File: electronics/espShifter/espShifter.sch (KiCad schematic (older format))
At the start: 114 parts, among them J1 Power In, J10 12V SENSE, J11 Motor A, J12 Motor E, J13 Motor I, J14 Motor B, J15 Motor F, J16 Motor J, J17 Motor C, J18 Motor G, J19 Motor K, J2 UART, J20 Motor D, J21 Motor H, J22 Motor L, J3 SENSOR, J4 IOVCC, J5 GND, J6 SR CHAIN IN, J7 SR CHAIN OUT, J8 RS485, J9 RS485, Q1 BSS138, Q2 BSS138, U1 Mega2560Shield, U10 ULN2003AModule, U11 INA219 Breakout Wide (blue), U12 ULN2003AModule, U13 ULN2003AModule, U14 ULN2003AModule, U15 ULN2003AModule, U16 LevelShifterModule, U17 RS485Module, U18 TTGO_TDisplay, U19 74HC244, U2 SSD1306_I2C, U20 74HC165, U21 74HC165, U22 ST7789_80x160, U23 D1_32, U24 74HC595, U25 74HC595, U26 74HC595, U27 74HC595, U28 74HC595, U29 74HC595, U3 ULN2003AModule, U30 ST7789_240x240, U31 INA219 Breakout Narrow (purpl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, U32 SP485, U33 INA219BxD, U34 TPL7407LA, U35 TPL7407LA, U36 TPL7407LA, U37 TPL7407LA, U38 TPL7407LA, U39 TPL7407LA, U4 ULN2003AModule, U40 TPL7407LA, U5 ULN2003AModule, U6 ULN2003AModule, U7 ULN2003AModule, U8 ULN2003AModule, U9 ULN2003AModule

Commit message: WIP ESP PCB
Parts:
- removed JP1: 12V_VIN, Connector_PinHeader_2.54mm:PinHeader_1x02_P2.54mm_Vertical, symbol Device:Jumper_NO_Small
- removed R10, R11, R12, R2, R3, R4, R5, R6, R7, R8, R9: 47k, Resistor_THT:R_Axial_DIN0204_L3.6mm_D1.6mm_P1.90mm_Vertical, symbol Device:R_Small
- removed U1: Mega2560Shield, Mega2560Shield:Mega2560Shield, symbol Mega2560Shield:Mega2560Shield
- removed U10, U12, U13, U14, U15, U3, U4, U5, U6, U7, U8, U9: ULN2003AModule, ULN2003AModule:ULN2003AModule, symbol ULN2003AModule:ULN2003AModule
- removed U17: RS485Module, RS485:RS485Module, symbol RS485Module:RS485Module
- added RN1, RN2, RN3: 47k, Resistor_SMD:R_Cat16-4, symbol Device:R_Pack04
- C1, C10, C11, C12, C13, C14, C15, C16, C17, C18, C19, C2, C20, C21, C22, C5, C6, C7, C8, C9: footprint (none) -> Capacitor_SMD:C_0805_2012Metric
- C3: footprint (none) -> Capacitor_SMD:CP_Elec_8x10.5
- C4: footprint (none) -> Capacitor_SMD:CP_Elec_4x5.4
- H1, H2, H3, H4: footprint MountingHole:MountingHole_4.3mm_M4_ISO7380 -> MountingHole:MountingHole_4.3mm_M4_ISO7380_Pad
- J1: footprint TerminalBlock:TerminalBlock_bornier-3_P5.08mm -> TerminalBlock:TerminalBlock_bornier-4_P5.08mm; symbol Connector:Screw_Terminal_01x03 -> Connector:Screw_Terminal_01x04
- J10, J8, J9: footprint (none) -> TerminalBlock:TerminalBlock_bornier-2_P5.08mm
- J4: value IOVCC -> 3.3v
- JP2: value RX 3.3V -> RX BYPASS
- JP3: value TX 3.3V -> TX BYPASS
- R1: value 47k -> 10k; footprint Resistor_THT:R_Axial_DIN0204_L3.6mm_D1.6mm_P1.90mm_Vertical -> Resistor_SMD:R_0805_2012Metric
- R13, R14, R15, R16, R17, R18: footprint Resistor_SMD:R_0805_2012Metric_Pad1.15x1.40mm_HandSolder -> Resistor_SMD:R_0805_2012Metric
- U19: footprint Package_DIP:DIP-20_W7.62mm -> Package_SO:TSSOP-20_4.4x6.5mm_P0.65mm
- U20, U21, U24, U25, U26, U27, U28, U29: footprint Package_DIP:DIP-16_W7.62mm -> Package_SO:SOIC-16_3.9x9.9mm_P1.27mm
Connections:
- net labels added: +3.3V
- net labels removed: IOVCC
- wire segments 980 -> 740
- no-connect marks 52 -> 35
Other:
- note removed: "47k. DNP for Mega 2560"
- note removed: "IOVCC is sourced by the MCU\nmodule that's inserted, at the\nappropriate IO voltage\n(3.3V or 5V)"
- note removed: "MCU Option 1: Mega2560 + SSD1306 OLED"
- note removed: "Motor Driver Modules"
- moved on the sheet: C1, C15, C16, C17, C18, C19, C20, C21, C22, J11, J12, J13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

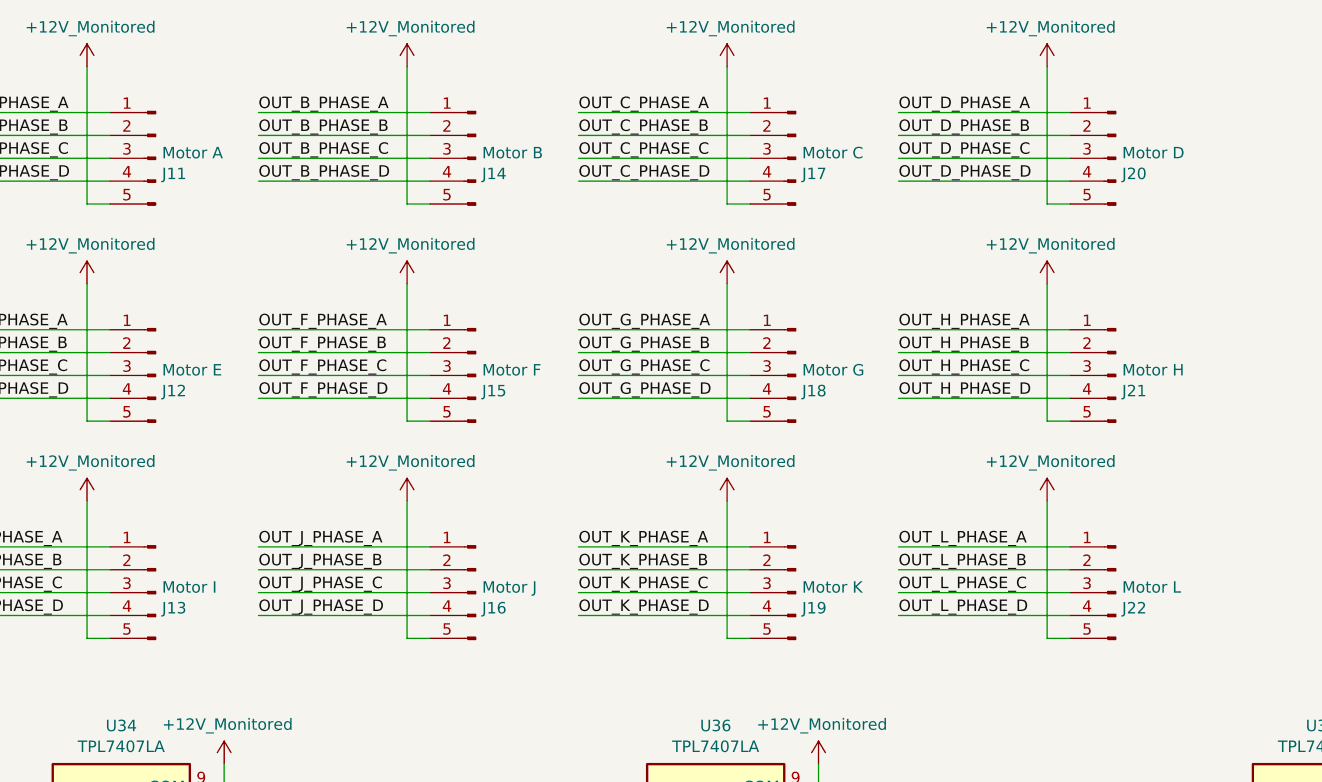
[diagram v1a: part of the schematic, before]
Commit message: WIP PCB Layout
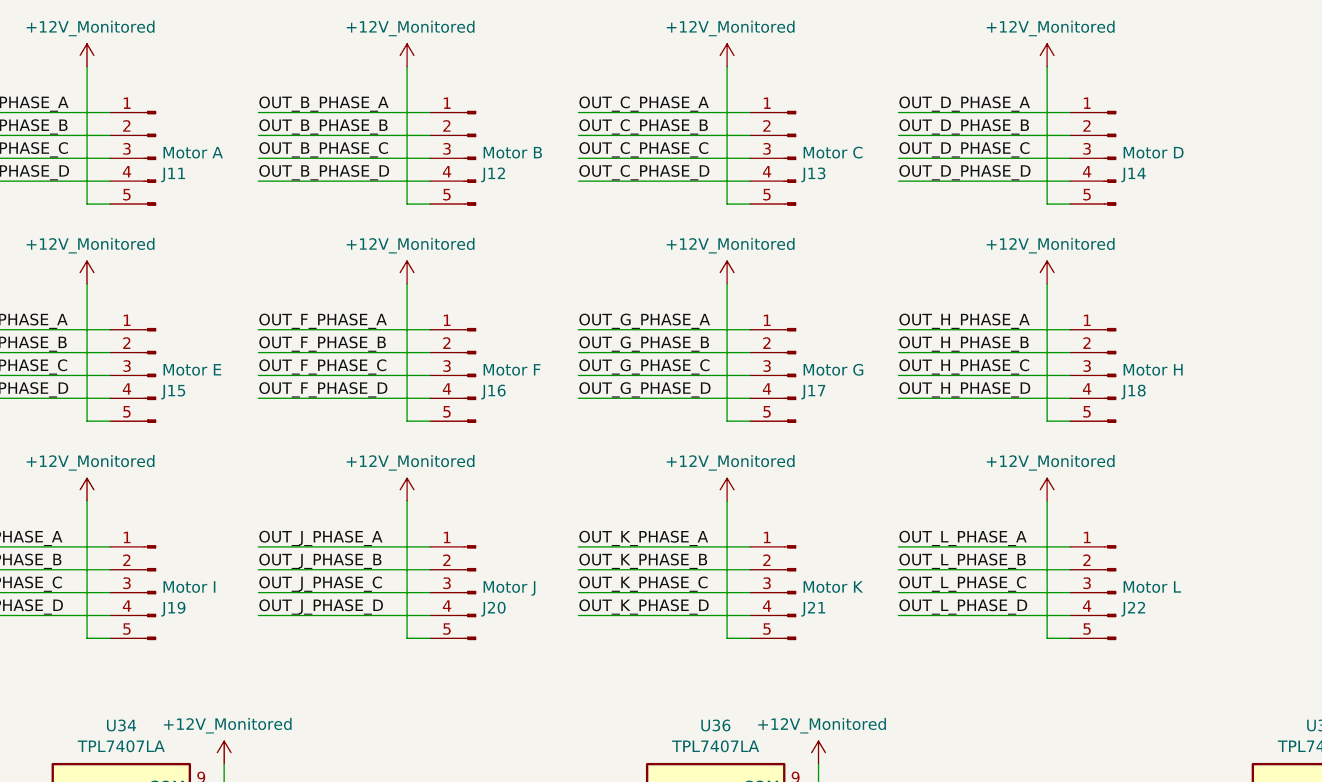
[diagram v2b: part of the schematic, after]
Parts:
- renumbered J14 to J12, J17 to J13, J20 to J14, J12 to J15, J15 to J16, J18 to J17, J21 to J18, J13 to J19, J16 to J20, J19 to J21
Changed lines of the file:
@@
 	2100 2750 2100 3350
 $Comp
-L Connector:Conn_01x05_Male J14
+L Connector:Conn_01x05_Male J12
 U 1 1 63D07061
 P 3800 3150
-F 0 "J14" H 3772 3082 50  0000 R CNN
+F 0 "J12" H 3772 3082 50  0000 R CNN
 F 1 "Motor B" H 3772 3173 50  0000 R CNN
 F 2 "JST_XH_Connectors:JST_XH_2-5mm_5pin" H 3800 3150 50  0001 C CNN
@@
 	3500 2750 3500 3350
 $Comp
-L Connector:Conn_01x05_Male J17
+L Connector:Conn_01x05_Male J13
 U 1 1 63DADADE
 P 5200 3150
-F 0 "J17" H 5172 3082 50  0000 R CNN
+F 0 "J13" H 5172 3082 50  0000 R CNN
 F 1 "Motor C" H 5172 3173 50  0000 R CNN
 F 2 "JST_XH_Connectors:JST_XH_2-5mm_5pin" H 5200 3150 50  0001 C CNN
@@
 	4900 2750 4900 3350
 $Comp
-L Connector:Conn_01x05_Male J20
+L Connector:Conn_01x05_Male J14
 U 1 1 63DADAFC
 P 6600 3150
-F 0 "J20" H 6572 3082 50  0000 R CNN
+F 0 "J14" H 6572 3082 50  0000 R CNN
 F 1 "Motor D" H 6572 3173 50  0000 R CNN
 F 2 "JST_XH_Connectors:JST_XH_2-5mm_5pin" H 6600 3150 50  0001 C CNN
@@
 	6300 2750 6300 3350
 $Comp
-L Connector:Conn_01x05_Male J12
+L Connector:Conn_01x05_Male J15
 U 1 1 63F11EEE
 P 2400 4100
-F 0 "J12" H 2372 4032 50  0000 R CNN
+F 0 "J15" H 2372 4032 50  0000 R CNN
 F 1 "Motor E" H 2372 4123 50  0000 R CNN
 F 2 "JST_XH_Connectors:JST_XH_2-5mm_5pin" H 2400 4100 50  0001 C CNN
@@
 	2100 3700 2100 4300
 $Comp
-L Connector:Conn_01x05_Male J15
+L Connector:Conn_01x05_Male J16
 U 1 1 63F11F0C
 P 3800 4100
-F 0 "J15" H 3772 4032 50  0000 R CNN
+F 0 "J16" H 3772 4032 50  0000 R CNN
 F 1 "Motor F" H 3772 4123 50  0000 R CNN
 F 2 "JST_XH_Connectors:JST_XH_2-5mm_5pin" H 3800 4100 50  0001 C CNN
@@
 	3500 3700 3500 4300
 $Comp
-L Connector:Conn_01x05_Male J18
+L Connector:Conn_01x05_Male J17
 U 1 1 63F11F2A
 P 5200 4100
-F 0 "J18" H 5172 4032 50  0000 R CNN
+F 0 "J17" H 5172 4032 50  0000 R CNN
 F 1 "Motor G" H 5172 4123 50  0000 R CNN
 F 2 "JST_XH_Connectors:JST_XH_2-5mm_5pin" H 5200 4100 50  0001 C CNN
@@
 	4900 3700 4900 4300
 $Comp
-L Connector:Conn_01x05_Male J21
+L Connector:Conn_01x05_Male J18
 U 1 1 63F11F48
 P 6600 4100
-F 0 "J21" H 6572 4032 50  0000 R CNN
+F 0 "J18" H 6572 4032 50  0000 R CNN
 F 1 "Motor H" H 6572 4123 50  0000 R CNN
 F 2 "JST_XH_Connectors:JST_XH_2-5mm_5pin" H 6600 4100 50  0001 C CNN
@@
 	6300 3700 6300 4300
 $Comp
-L Connector:Conn_01x05_Male J13
+L Connector:Conn_01x05_Male J19
 U 1 1 63FD55F8
 P 2400 5050
-F 0 "J13" H 2372 4982 50  0000 R CNN
+F 0 "J19" H 2372 4982 50  0000 R CNN
 F 1 "Motor I" H 2372 5073 50  0000 R CNN
 F 2 "JST_XH_Connectors:JST_XH_2-5mm_5pin" H 2400 5050 50  0001 C CNN
@@
 	2100 4650 2100 5250
 $Comp
-L Connector:Conn_01x05_Male J16
+L Connector:Conn_01x05_Male J20
 U 1 1 63FD5616
 P 3800 5050
-F 0 "J16" H 3772 4982 50  0000 R CNN
+F 0 "J20" H 3772 4982 50  0000 R CNN
 F 1 "Motor J" H 3772 5073 50  0000 R CNN
 F 2 "JST_XH_Connectors:JST_XH_2-5mm_5pin" H 3800 5050 50  0001 C CNN
@@
 	3500 4650 3500 5250
 $Comp
-L Connector:Conn_01x05_Male J19
+L Connector:Conn_01x05_Male J21
 U 1 1 63FD5634
 P 5200 5050
-F 0 "J19" H 5172 4982 50  0000 R CNN
+F 0 "J21" H 5172 4982 50  0000 R CNN
 F 1 "Motor K" H 5172 5073 50  0000 R CNN
 F 2 "JST_XH_Connectors:JST_XH_2-5mm_5pin" H 5200 5050 50  0001 C CNN
